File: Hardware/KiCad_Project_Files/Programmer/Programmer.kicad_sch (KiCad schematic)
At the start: 24 parts, among them J1 USB_C_Receptacle_USB2.0, J2 R_PI_4, J3 SWD, Q1 FDN335N, U1 MIC5205-3.3YM5, U2 ATSAMD21G18A-A, Y1 32.876

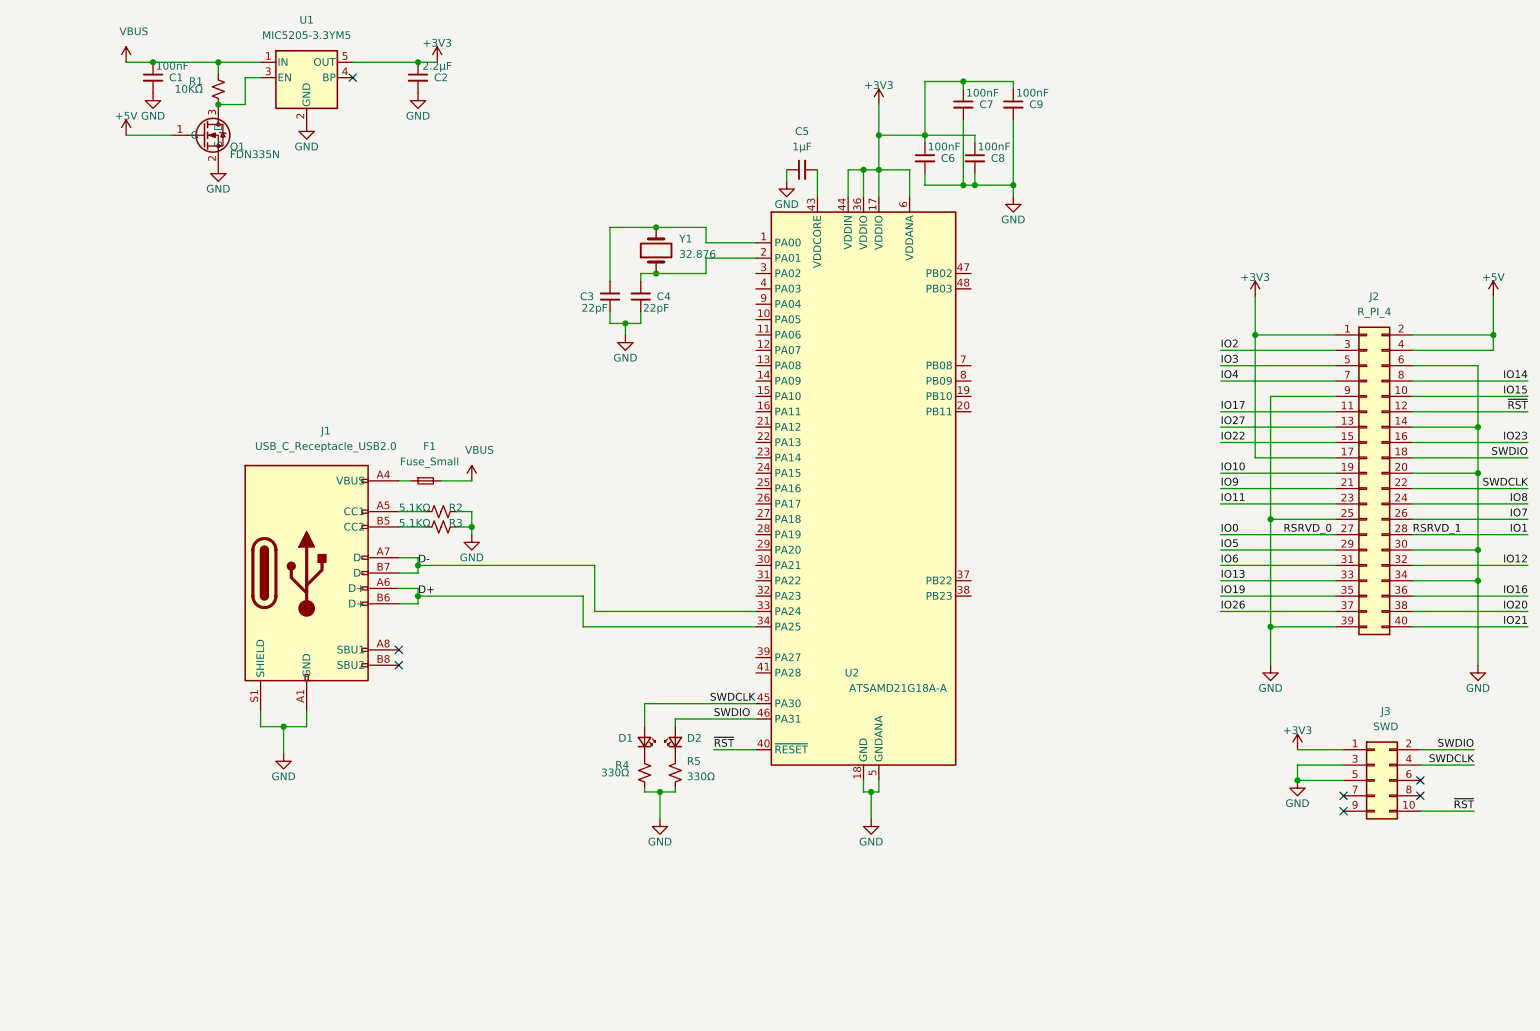
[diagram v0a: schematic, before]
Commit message: layout init
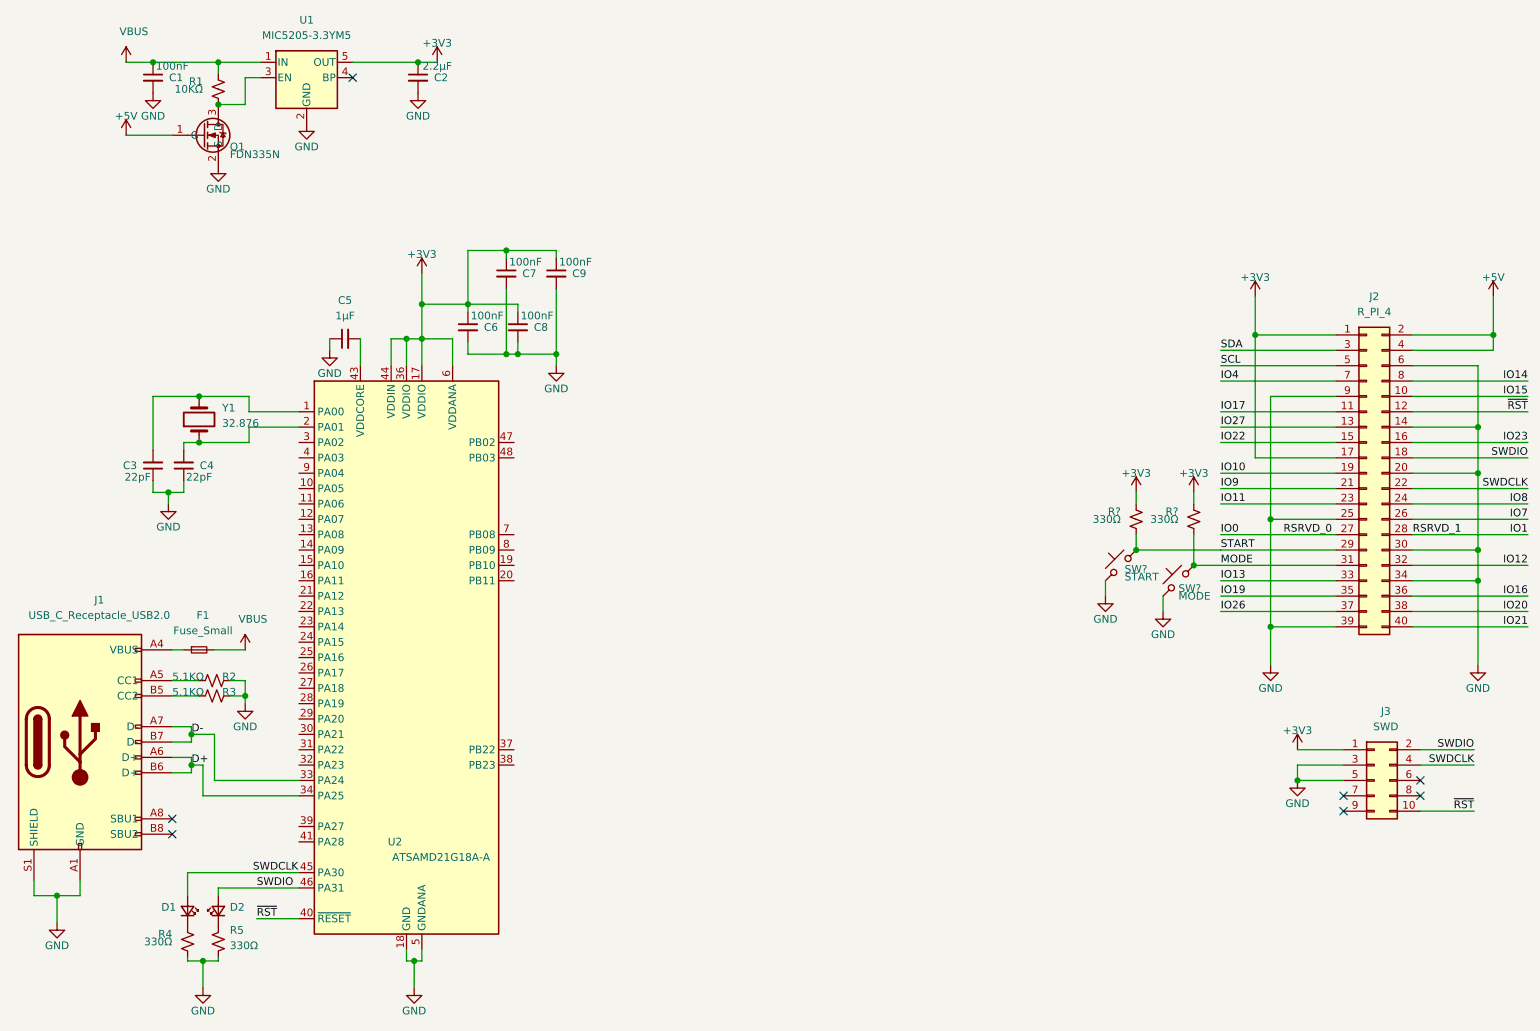
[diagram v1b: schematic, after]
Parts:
- added R? (x2): 330Ω, Resistor_SMD:R_0603_1608Metric, symbol Device:R_Small_US
- added SW?: START, Button_Switch_SMD:SW_SPST_TL3342, symbol Switch:SW_Push_45deg
- added SW?: MODE, Button_Switch_SMD:SW_SPST_TL3342, symbol Switch:SW_Push_45deg
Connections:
- net +3V3: now also R?.1, R?.1
- net GND: now also SW?.1, SW?.1
- net IO2 renamed SDA
- net IO3 renamed SCL
- net IO5 renamed START
- net START: now also R?.2, SW?.2
- net IO6 renamed MODE
- net MODE: now also R?.2, SW?.2
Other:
- moved on the sheet: C3, C4, C5, C6, C7, C8, C9, D1, D2, F1, J1, R2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
